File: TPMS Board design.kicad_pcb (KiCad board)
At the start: 2 copper layers, 22 parts, among them J1 CAN_IN, J2 CAN_OUT, J3 CAN_DB9, U1 ADM3055E, U2 ESP32-C3, U3 CDSOT23-T24CAN, Y1 Crystal

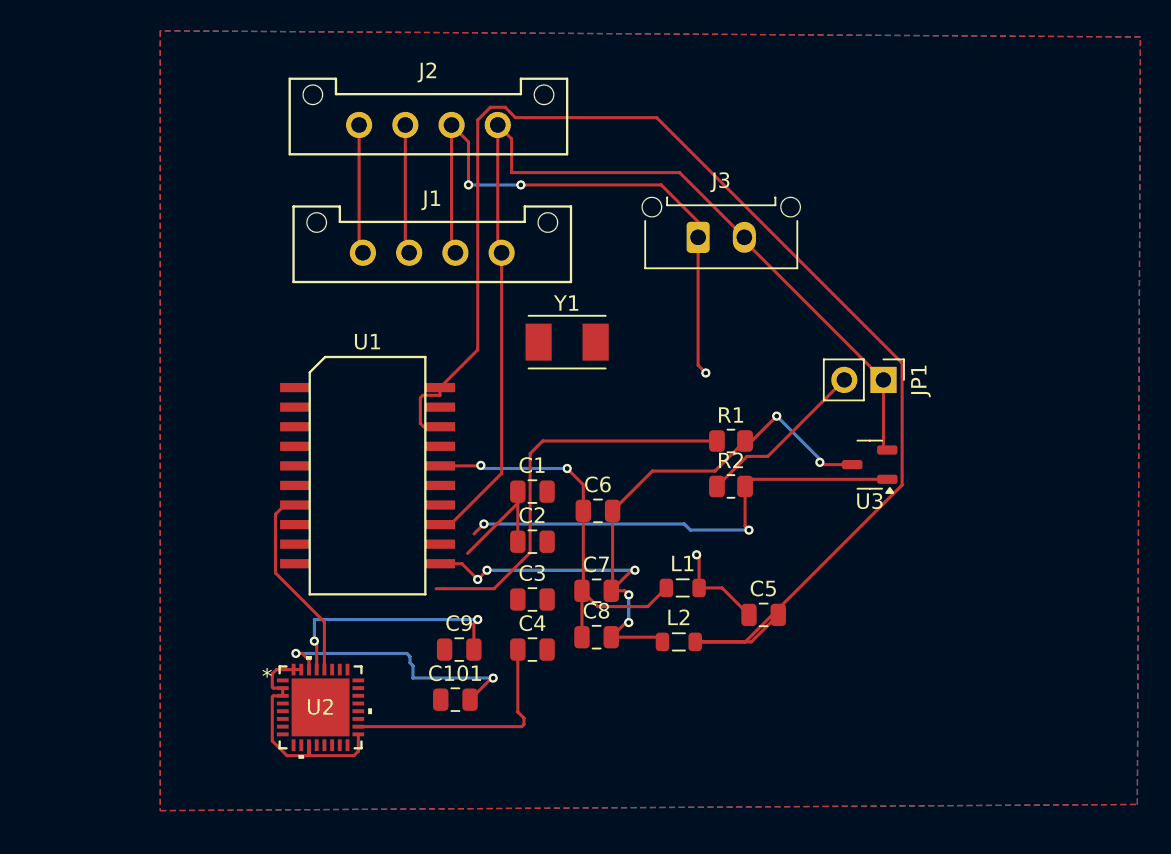
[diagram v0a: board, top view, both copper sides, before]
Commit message: IC
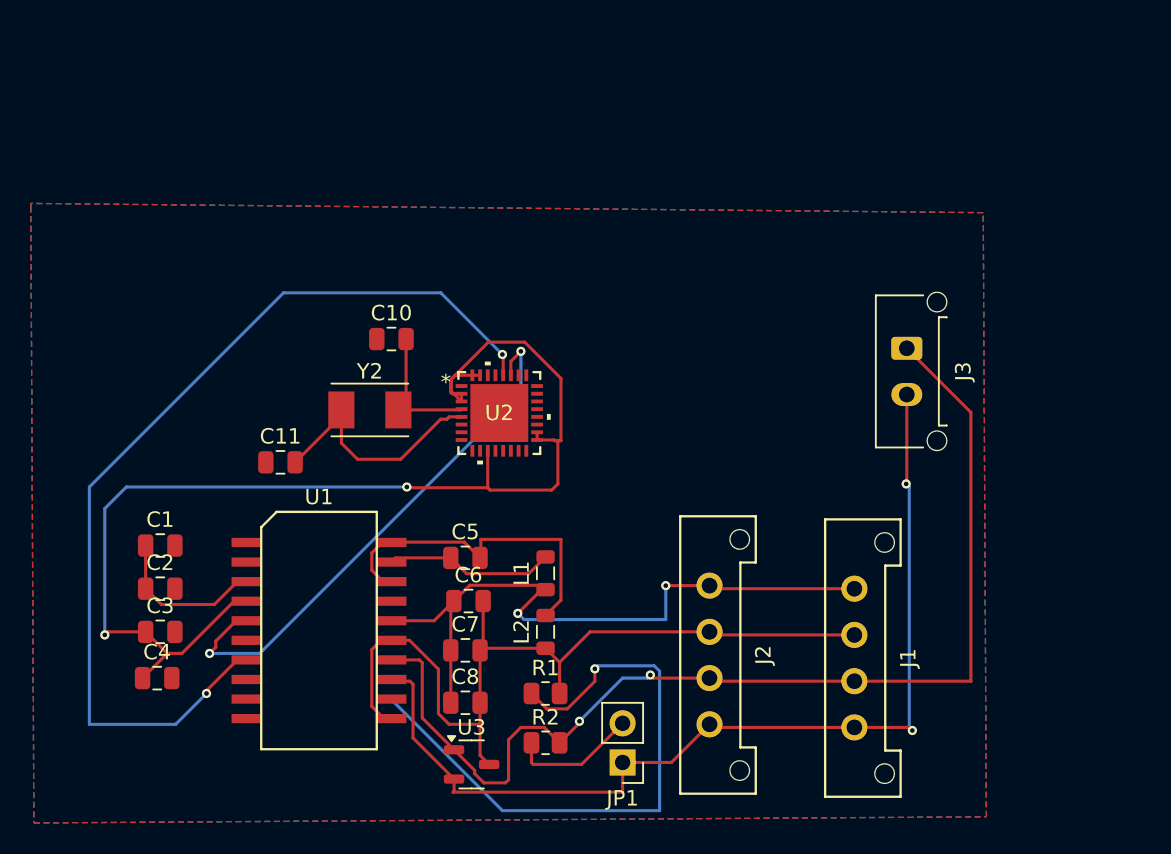
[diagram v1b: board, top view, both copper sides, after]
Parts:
- removed C101: 18pf, Capacitor_SMD:C_0805_2012Metric
- removed C9: 18Pf, Capacitor_SMD:C_0805_2012Metric
- removed Y1: Crystal, Crystal:Crystal_SMD_TXC_7A-2Pin_5x3.2mm
- added C10: 18Pf, Capacitor_SMD:C_0805_2012Metric, F.Cu at (128.6, 73.6)
- added C11: 18pf, Capacitor_SMD:C_0805_2012Metric, F.Cu at (121.4, 81.6)
- added Y2: Crystal, Crystal:Crystal_SMD_TXC_7A-2Pin_5x3.2mm, F.Cu at (127.2, 78.2)
- moved J1 38.6 mm to (158.6, 89.8), turned to -90 degrees
- moved J2 37.6 mm to (149.2, 89.6), turned to -90 degrees
- moved U3 32.3 mm to (133.8, 101.2), turned to 0 degrees
- moved JP1 30.0 mm to (143.6, 101.1), turned to 180 degrees
- moved C4 24.4 mm to (113.4, 95.6)
- moved C1 24.4 mm to (113.6, 87.0)
- moved C2 24.3 mm to (113.6, 89.8)
- moved C3 24.2 mm to (113.6, 92.6)
- moved U2 22.3 mm to (135.6, 78.4)
- moved R2 20.5 mm to (138.6, 99.8)
- moved R1 20.3 mm to (138.6, 96.6)
- moved C5 19.7 mm to (133.4, 87.8)
- moved J3 15.3 mm to (162.0, 74.2), turned to -90 degrees
- moved U1 10.5 mm to (123.9, 92.5)
- moved C6 10.2 mm to (133.6, 90.6)
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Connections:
- C3 pad 1: +3V3 -> +3.3V
- C4 pad 1: +3V3 -> +3.3V
- U1 pad 4: +3V3 -> +3.3V
- U2 pad 11: +3V3 -> +3.3V
- U2 pad 17: +3V3 -> +3.3V
- U2 pad 18: +3V3 -> +3.3V
- U2 pad 2: +3V3 -> +3.3V
- U2 pad 29: Net-(U2-XTAL_N) -> unconnected-(U2-XTAL_N-Pad29)
- U2 pad 3: +3V3 -> +3.3V
- U2 pad 30: Net-(U2-XTAL_P) -> unconnected-(U2-XTAL_P-Pad30)
- U2 pad 31: +3V3 -> +3.3V
- U2 pad 32: +3V3 -> +3.3V
- U2 pad 4: unconnected-(U2-GPIO0/XTAL_32K_P-Pad4) -> Net-(U2-GPIO0/XTAL_32K_P)
- U2 pad 5: unconnected-(U2-GPIO1/XTAL_32K_N-Pad5) -> Net-(U2-GPIO1/XTAL_32K_N)
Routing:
- net +3.3V: track 0.00 -> 78.2 mm, vias 0 -> 2
- net Net-(C5-Pad2): track 89.7 -> 22.2 mm
- net Net-(U1-TX): track 12.9 -> 62.5 mm, vias 0 -> 2
- net Net-(U1-RX): track 0.00 -> 35.2 mm, vias 0 -> 2
- net +3V3: track 32.6 -> 0.00 mm
- net Net-(U2-XTAL_P): track 17.9 -> 0.00 mm, vias 2 -> 0
- net Net-(U2-GPIO1/XTAL_32K_N): track 0.00 -> 16.2 mm
- net Net-(U2-XTAL_N): track 16.0 -> 0.00 mm, vias 2 -> 0
- net /RSlope: track 26.0 -> 39.9 mm, vias 0 -> 1
- net Net-(J1-Pin_1): track 35.2 -> 44.5 mm
- net Net-(U2-GPIO0/XTAL_32K_P): track 0.00 -> 8.93 mm
- net Net-(U1-V_ISO_Out): track 6.18 -> 11.0 mm, vias 1 -> 0
- net /TERM_H: track 11.1 -> 8.35 mm
- net Net-(J1-Pin_2): track 57.5 -> 55.1 mm, vias 7 -> 0
- net /CAN_H: track 69.9 -> 71.9 mm, vias 5 -> 2
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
